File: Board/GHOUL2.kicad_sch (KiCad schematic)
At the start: 15 parts, among them Q1 IRF540N, Q2 IRF540N, U1 Teensy3.5_All_Pins, U10 GHOULIMU, U2 LM7805_TO220, U3 BMP280, U4 Feedback_Serv, U5 LM1084-ADJ, U6 NichromeConnector, U7 Ultimate_GPS_Breakout_v3, U8 Xbee, U9 NichromeConnector

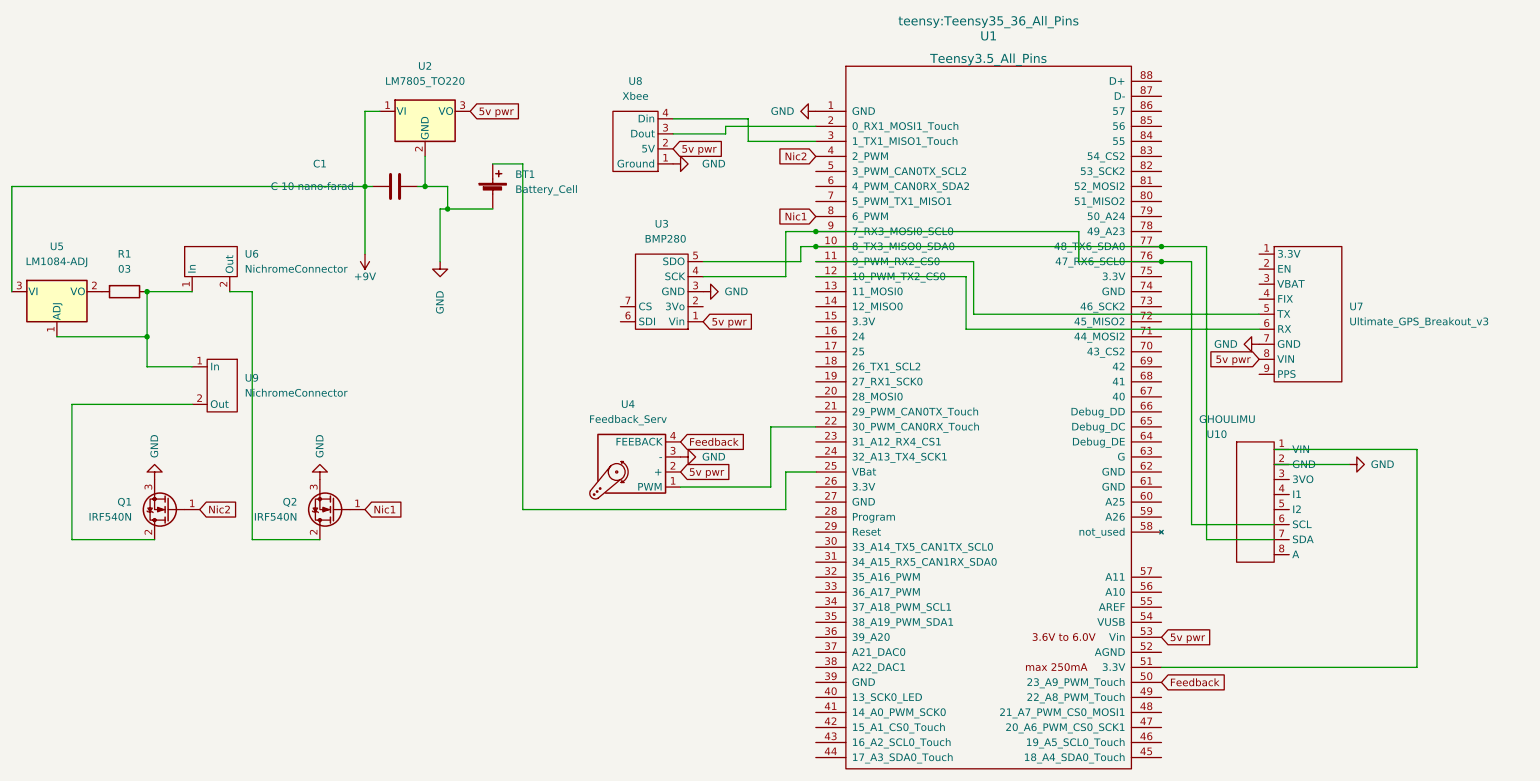
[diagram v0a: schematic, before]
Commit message: did a layout, needs some more work but at least it exists now
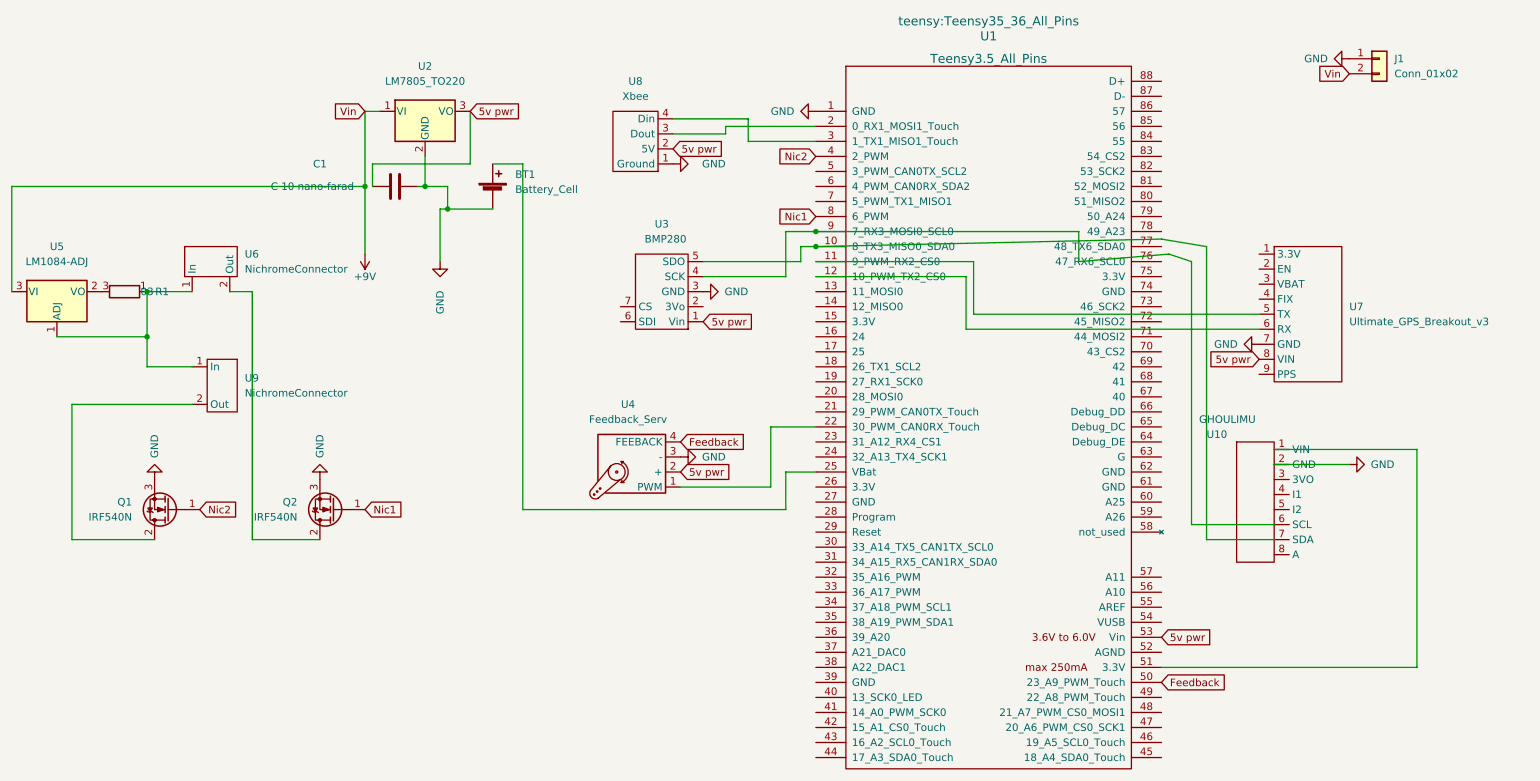
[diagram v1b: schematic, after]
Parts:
- added J1: Conn_01x02, Connector_AMASS:AMASS_XT30PW-M_1x02_P2.50mm_Horizontal, symbol Connector_Generic:Conn_01x02
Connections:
- net +9V: now also J1.2 (Pin_2); no longer C1.1
- net 5v pwr: now also C1.1
- net GND: now also J1.1 (Pin_1)
- net at U5.2 (VO): now also R1.3; no longer R1.2
- net at U1.9 (7_RX3_MOSI0_SCL0), U10.6 (SCL), U3.4 (SCK): no longer U1.76 (47_RX6_SCL0)
- net at U1.10 (8_TX3_MISO0_SDA0), U10.7 (SDA), U3.5 (SDO): no longer U1.77 (48_TX6_SDA0)
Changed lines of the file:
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@@
   (junction (at 96.52 53.34) (diameter 0) (color 0 0 0 0)
   )
-  (junction (at 231.14 63.5) (diameter 0) (color 0 0 0 0)
-  )
   (junction (at 59.69 78.74) (diameter 0) (color 0 0 0 0)
   )
@@
   (junction (at 110.49 57.15) (diameter 0) (color 0 0 0 0)
   )
-  (junction (at 231.14 66.04) (diameter 0) (color 0 0 0 0)
-  )
   (junction (at 59.69 71.12) (diameter 0) (color 0 0 0 0)
   )
@@
     (stroke (width 0) (type default) (color 0 0 0 0))
   )
+  (wire (pts (xy 97.79 53.34) (xy 97.79 49.53))
+    (stroke (width 0) (type default) (color 0 0 0 0))
+  )
   (wire (pts (xy 247.65 77.47) (xy 198.12 77.47))
     (stroke (width 0) (type default) (color 0 0 0 0))
@@
   )
   (wire (pts (xy 250.19 113.03) (xy 238.76 113.03))
+    (stroke (width 0) (type default) (color 0 0 0 0))
+  )
+  (wire (pts (xy 97.79 49.53) (xy 114.3 49.53))
     (stroke (width 0) (type default) (color 0 0 0 0))
   )
@@
     (stroke (width 0) (type default) (color 0 0 0 0))
   )
-  (wire (pts (xy 231.14 66.04) (xy 236.22 66.04))
+  (wire (pts (xy 232.41 64.77) (xy 236.22 66.04))
     (stroke (width 0) (type default) (color 0 0 0 0))
   )
@@
     (stroke (width 0) (type default) (color 0 0 0 0))
   )
+  (wire (pts (xy 114.3 49.53) (xy 114.3 40.64))
+    (stroke (width 0) (type default) (color 0 0 0 0))
+  )
   (wire (pts (xy 96.52 40.64) (xy 99.06 40.64))
     (stroke (width 0) (type default) (color 0 0 0 0))
@@
     (stroke (width 0) (type default) (color 0 0 0 0))
   )
-  (wire (pts (xy 172.72 63.5) (xy 231.14 63.5))
+  (wire (pts (xy 172.72 63.5) (xy 231.14 62.23))
     (stroke (width 0) (type default) (color 0 0 0 0))
   )
@@
     (stroke (width 0) (type default) (color 0 19 255 1))
   )
-  (wire (pts (xy 96.52 53.34) (xy 97.79 53.34))
-    (stroke (width 0) (type default) (color 0 0 0 0))
-  )
   (wire (pts (xy 59.69 78.74) (xy 59.69 71.12))
     (stroke (width 0) (type default) (color 0 0 0 0))
@@
     (stroke (width 0) (type default) (color 0 0 0 0))
   )
-  (wire (pts (xy 217.17 66.04) (xy 231.14 66.04))
+  (wire (pts (xy 217.17 66.04) (xy 232.41 64.77))
     (stroke (width 0) (type default) (color 0 0 0 0))
   )
@@
     (stroke (width 0) (type default) (color 0 0 0 0))
   )
-  (wire (pts (xy 231.14 63.5) (xy 238.76 63.5))
+  (wire (pts (xy 231.14 62.23) (xy 238.76 63.5))
     (stroke (width 0) (type default) (color 0 0 0 0))
   )
@@
     )
   )
+  (global_label "Vin" (shape input) (at 96.52 40.64 180) (fields_autoplaced)
+    (effects (font (size 1.27 1.27)) (justify right))
+    (property "Intersheet References" "${INTERSHEET_REFS}" (id 0) (at 91.2645 40.5606 0)
+      (effects (font (size 1.27 1.27)) (justify right) hide)
+    )
+  )
   (global_label "5v pwr" (shape input) (at 114.3 40.64 0) (fields_autoplaced)
     (effects (font (size 1.27 1.27)) (justify left))
@@
     (property "Intersheet References" "${INTERSHEET_REFS}" (id 0) (at 103.1664 107.8706 0)
       (effects (font (size 1.27 1.27)) (justify left) hide)
+    )
+  )
+  (global_label "Vin" (shape input) (at 262.89 34.29 180) (fields_autoplaced)
+    (effects (font (size 1.27 1.27)) (justify right))
+    (property "Intersheet References" "${INTERSHEET_REFS}" (id 0) (at 257.6345 34.2106 0)
+      (effects (font (size 1.27 1.27)) (justify right) hide)
     )
   )
@@
   (symbol (lib_id "Device:R") (at 55.88 71.12 270) (unit 1)
     (in_bom yes) (on_board yes) (fields_autoplaced)
-    (property "Reference" "R1" (id 0) (at 55.88 64.77 90))
-    (property "Value" "03" (id 1) (at 55.88 67.31 90))
-    (property "Footprint" "Package_TO_SOT_SMD:TO-263-2" (id 2) (at 55.88 69.342 90)
+    (property "Reference" "R1" (id 0) (at 62.23 71.12 90))
+    (property "Value" "03" (id 1) (at 59.69 71.12 90))
+    (property "Footprint" "Package_TO_SOT_SMD:TO-263-2" (id 2) (at 57.658 71.12 90)
       (effects (font (size 1.27 1.27)) hide)
     )
@@
     )
     (pin "1")
-    (pin "2")
+    (pin "3")
   )
   (symbol (lib_id "power:GND") (at 172.72 40.64 270) (unit 1)
@@
     (pin "3")
     (pin "4")
+  )
+  (symbol (lib_id "power:GND") (at 262.89 31.75 270) (unit 1)
+    (in_bom yes) (on_board yes)
+    (property "Reference" "#PWR0111" (id 0) (at 256.54 31.75 0)
+      (effects (font (size 1.27 1.27)) hide)
+    )
+    (property "Value" "GND" (id 1) (at 255.27 31.75 90)
+      (effects (font (size 1.27 1.27)) (justify left))
+    )
+    (property "Footprint" "" (id 2) (at 262.89 31.75 0)
+      (effects (font (size 1.27 1.27)) hide)
+    )
+    (property "Datasheet" "" (id 3) (at 262.89 31.75 0)
+      (effects (font (size 1.27 1.27)) hide)
+    )
+    (pin "1")
   )
   (symbol (lib_id "GHOUL:NichromeConnector") (at 69.85 68.58 0) (unit 1)
@@
     )
     (pin "1")
+  )
+  (symbol (lib_id "Connector_Generic:Conn_01x02") (at 267.97 31.75 0) (unit 1)
+    (in_bom yes) (on_board yes) (fields_autoplaced)
+    (property "Reference" "J1" (id 0) (at 270.51 31.7499 0)
+      (effects (font (size 1.27 1.27)) (justify left))
+    )
+    (property "Value" "Conn_01x02" (id 1) (at 270.51 34.2899 0)
+      (effects (font (size 1.27 1.27)) (justify left))
+    )
+    (property "Footprint" "Connector_AMASS:AMASS_XT30PW-M_1x02_P2.50mm_Horizontal" (id 2) (at 267.97 31.75 0)
+      (effects (font (size 1.27 1.27)) hide)
+    )
+    (property "Datasheet" "~" (id 3) (at 267.97 31.75 0)
+      (effects (font (size 1.27 1.27)) hide)
+    )
+    (pin "1")
+    (pin "2")
   )
   (symbol (lib_id "power:GND") (at 149.86 99.06 90) (unit 1)
@@
       (reference "#PWR0110") (unit 1) (value "GND") (footprint "")
     )
+    (path "/707fed9e-5b9e-40a5-a3f5-afb695484dbb"
+      (reference "#PWR0111") (unit 1) (value "GND") (footprint "")
+    )
     (path "/e100fb02-ae0f-4575-a8f0-e7fb3c16a01e"
       (reference "BT1") (unit 1) (value "Battery_Cell") (footprint "Battery:BatteryHolder_Keystone_3000_1x12mm")
@@
       (reference "C1") (unit 1) (value "C 10 nano-farad") (footprint "GHOULFootPrints:GhoulResistor")
     )
+    (path "/9902bfe6-8d4f-44df-947a-5e52f92861a4"
+      (reference "J1") (unit 1) (value "Conn_01x02") (footprint "Connector_AMASS:AMASS_XT30PW-M_1x02_P2.50mm_Horizontal")
+    )
     (path "/2fd90422-ba41-4885-811c-3484a05fc047"
